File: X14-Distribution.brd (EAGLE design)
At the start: 152.4 x 76.2 mm, 57 parts, among them Q1 310mA/60V/1.6Ω, Q2 IRF1018EPBF, Q3 IRF1018EPBF, Q4 IRF1018EPBF, Q5 IRLML5203, Q6 IRLML5203, Q7 IRLML5203, Q8 IRLML5203, U1 DIST_OR_CONTROL_ALTMK06A-M, U2 DIST_OR_CONTROL_ALTMK06A-M

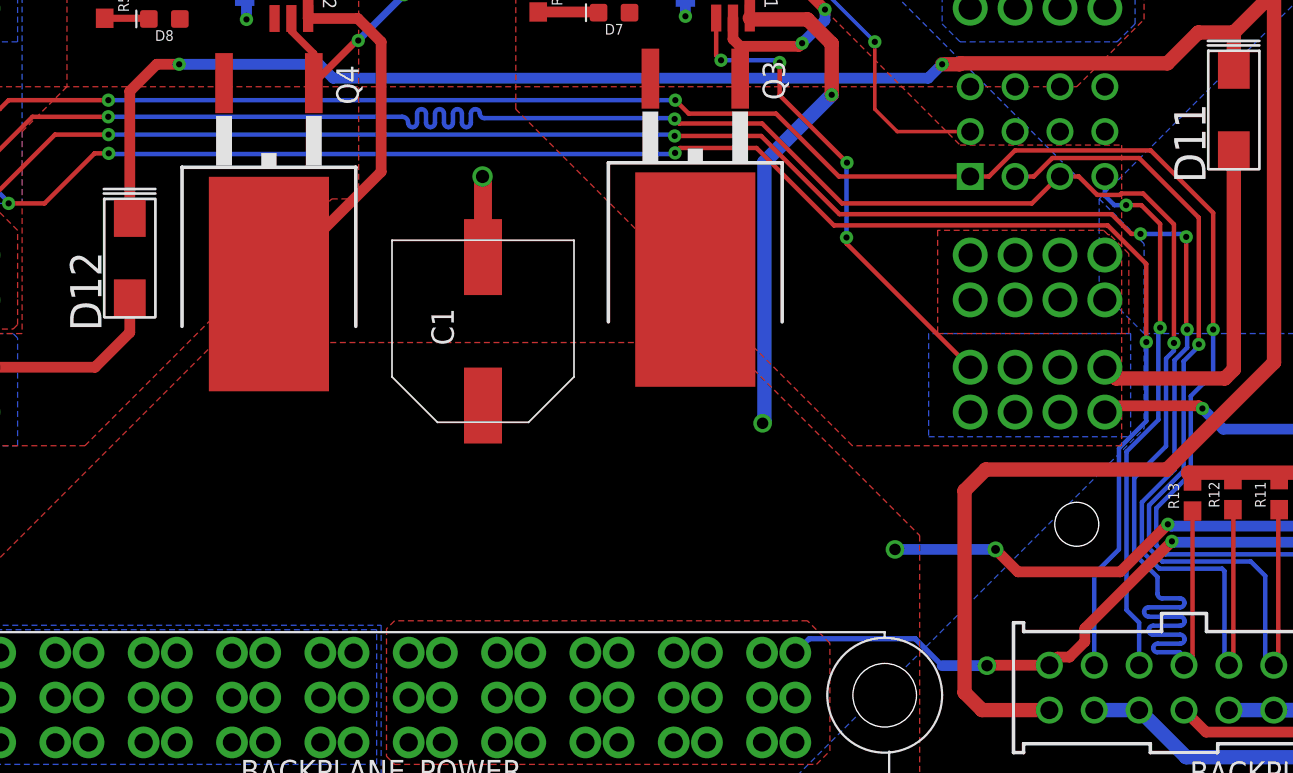
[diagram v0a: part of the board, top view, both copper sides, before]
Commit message: Changed curves back to zigzagy thingys
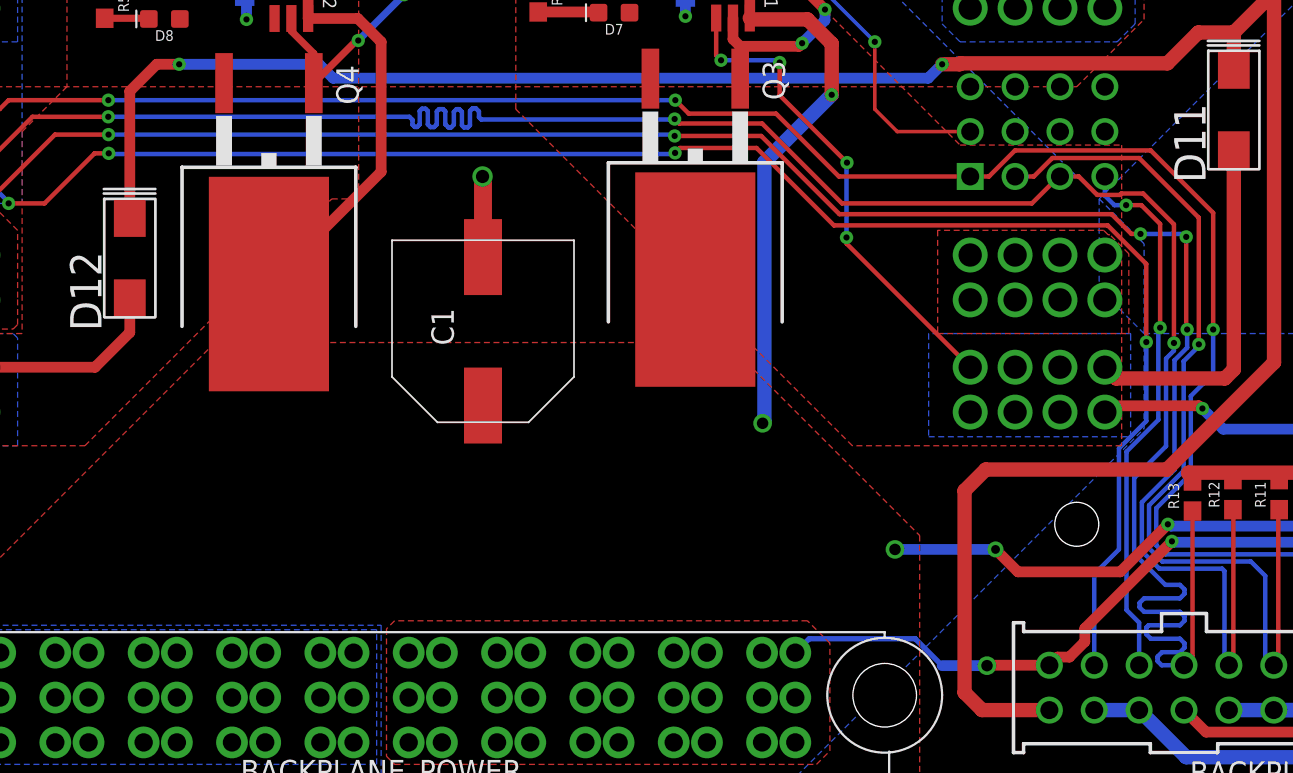
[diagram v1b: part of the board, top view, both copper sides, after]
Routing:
- net CLK: track 127.6 -> 129.5 mm
